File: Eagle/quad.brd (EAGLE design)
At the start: 100 x 60 mm, 20 parts

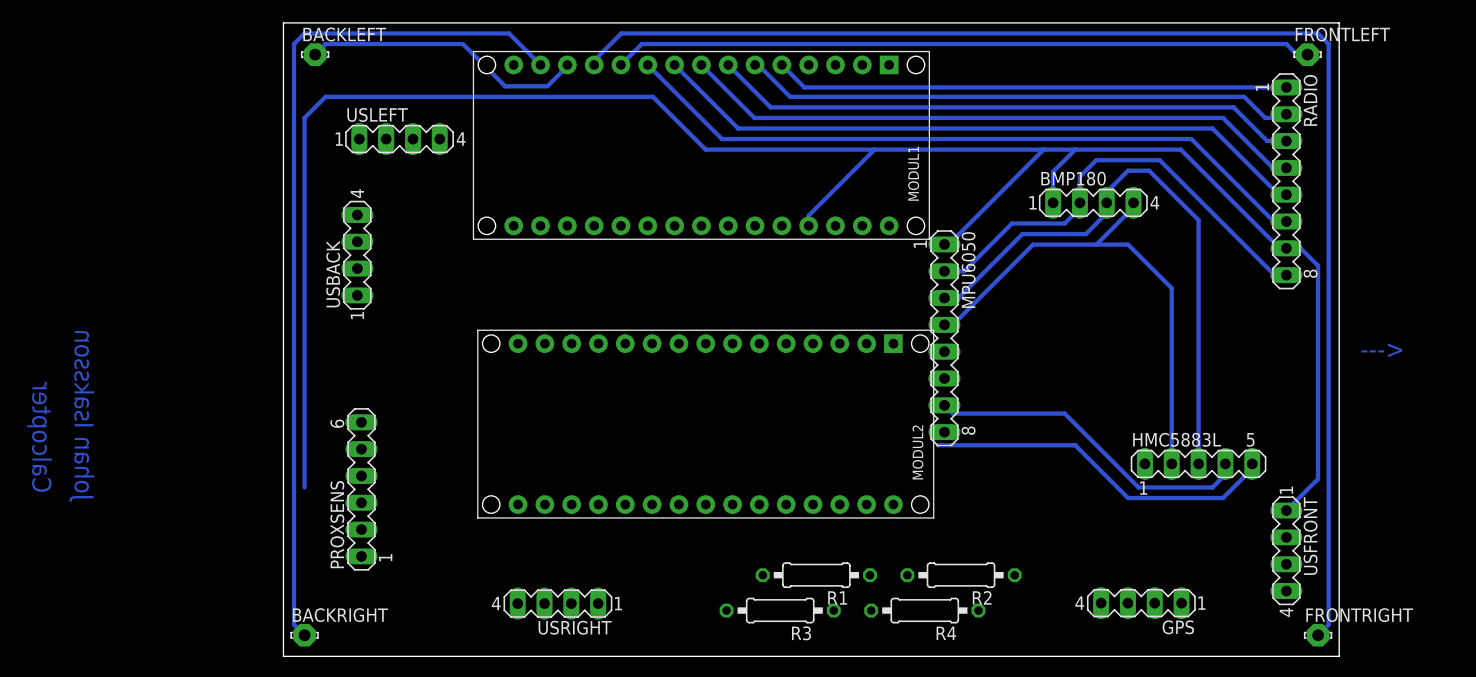
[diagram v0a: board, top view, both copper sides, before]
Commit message: Large board done
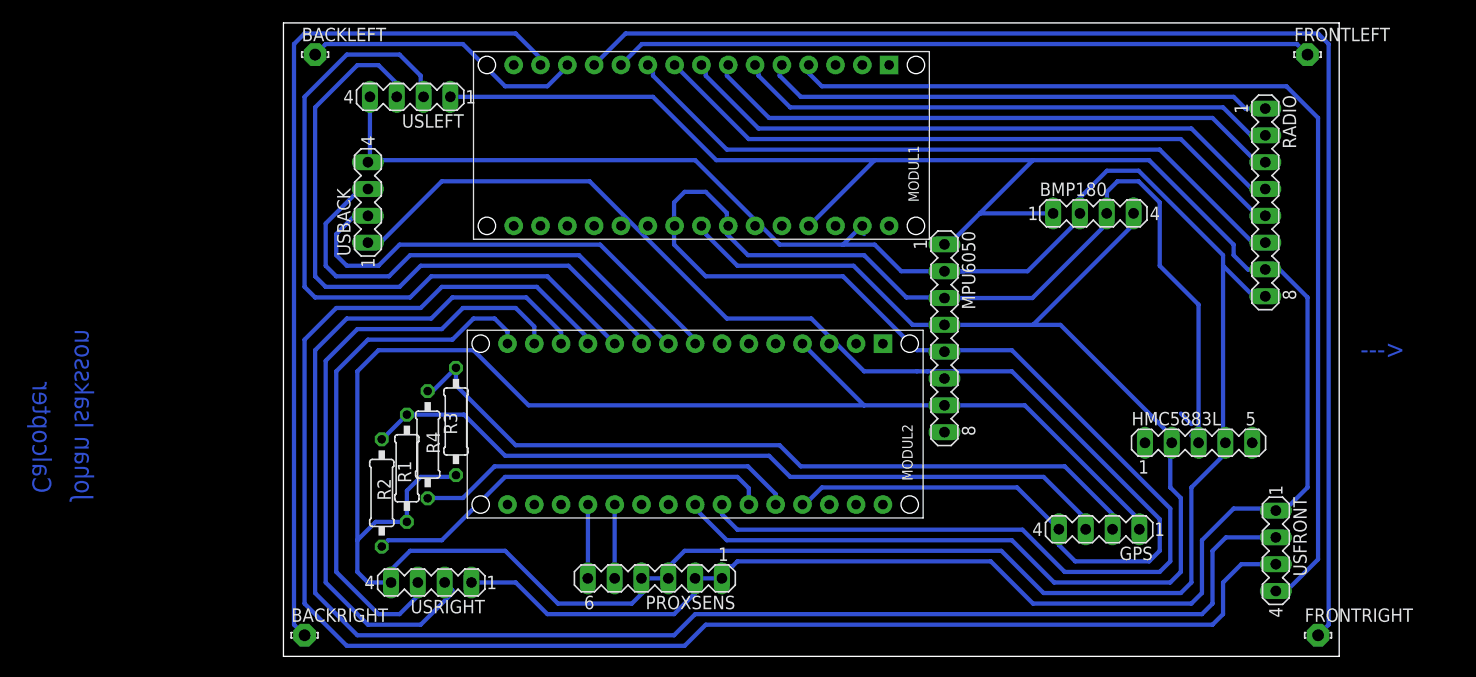
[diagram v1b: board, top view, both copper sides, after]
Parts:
- moved R2 53.5 mm to (11.7, 17.8), turned to 90 degrees
- moved R4 47.9 mm to (16.3, 22.2), turned to 90 degrees
- moved R1 41.9 mm to (9.31, 15.5), turned to 270 degrees
- moved R3 36.9 mm to (13.7, 20.1), turned to 270 degrees
- moved PROXSENS 29.0 mm to (35.2, 7.39), turned to 180 degrees
- moved USRIGHT 12.2 mm to (14.0, 7.00)
- moved GPS 8.06 mm to (77.3, 12.0)
- moved USBACK 5.10 mm to (8.00, 43.0)
- moved USLEFT 4.12 mm to (12.0, 53.0), turned to 180 degrees
- moved RADIO 2.83 mm to (93.0, 43.0)
- moved HMC5883L 2.00 mm to (86.7, 20.2)
- moved BMP180 1.00 mm to (76.7, 42.0)
- moved MODUL2 1.00 mm to (39.0, 22.0)
- moved USFRONT 1.00 mm to (94.0, 10.0)
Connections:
- removed net N$26 (its old number): MODUL2.J1.9, USRIGHT.2
- removed net N$27: MODUL2.J1.10, USRIGHT.3
- removed net N$30: MODUL2.J1.11, USBACK.2
- new net N$2: MODUL2.J1.11, USLEFT.2
- new net N$28: MODUL2.J1.10, USLEFT.3
- new net N$32: MODUL2.J1.9, USBACK.3
- net N$22: now also MODUL2.J1.8, USBACK.2; no longer MODUL2.J1.7, USFRONT.2
- net N$23: now also MODUL2.J1.15, USRIGHT.3; no longer MODUL2.J1.8, USFRONT.3
- net N$24: now also MODUL2.J1.14, USRIGHT.2; no longer MODUL2.J1.5, USLEFT.2
- net N$25: now also MODUL2.J1.13, USFRONT.2; no longer MODUL2.J1.6, USLEFT.3
- net N$29: now also USFRONT.3; no longer USBACK.3
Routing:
- net N$9: track 74.5 -> 456.0 mm
- net N$26: track 191.7 -> 361.0 mm
- net N$29: track 0.00 -> 155.2 mm
- net N$25: track 0.00 -> 151.0 mm
- net N$16: track 55.3 -> 198.1 mm
- net N$17: track 49.2 -> 130.5 mm
- net N$21: track 0.00 -> 74.3 mm
- net N$20: track 0.00 -> 72.7 mm
- net N$2: track 0.00 -> 67.4 mm
- net N$28: track 0.00 -> 63.1 mm
- net N$24: track 0.00 -> 61.4 mm
- net N$23: track 0.00 -> 50.6 mm
- net N$32: track 0.00 -> 46.5 mm
- net N$22: track 0.00 -> 45.3 mm
- net N$18: track 0.00 -> 39.5 mm
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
